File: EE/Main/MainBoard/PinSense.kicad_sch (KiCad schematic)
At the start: 15 parts, among them U10 DRV5032AJDBZR, U6 DRV5032AJDBZR, U7 DRV5032AJDBZR, U8 DRV5032AJDBZR, U9 DRV5032AJDBZR

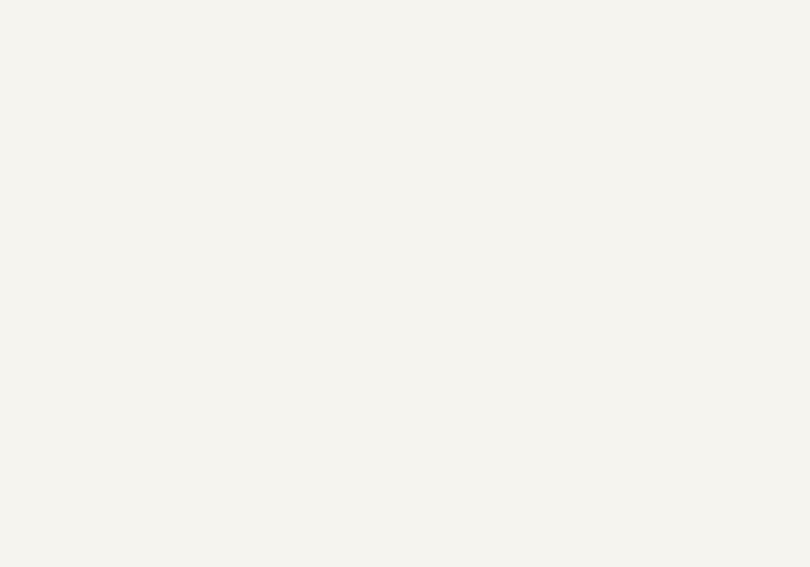
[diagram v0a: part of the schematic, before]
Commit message: Potential Revision
Potentially fabb-able rev.
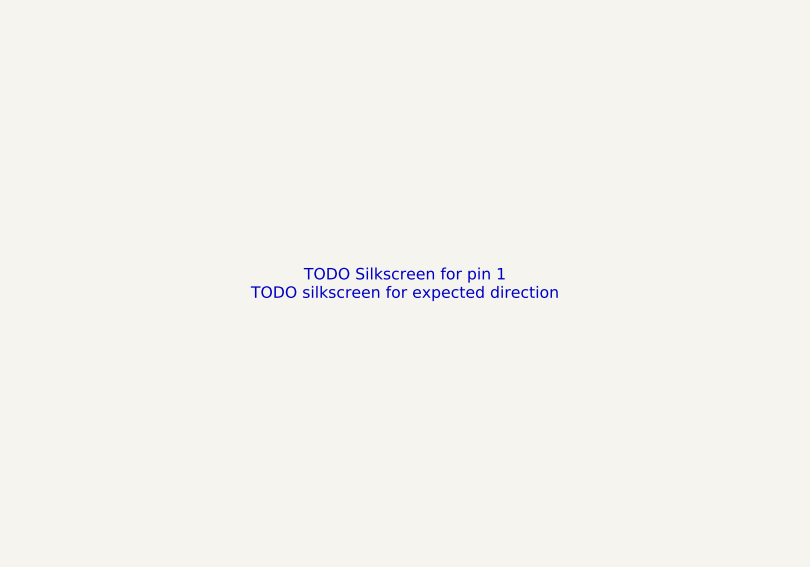
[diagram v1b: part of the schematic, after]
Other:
- note added: "TODO Silkscreen for pin 1 TODO silkscreen for expected direction"
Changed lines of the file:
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@@
 		(at 133.858 114.3)
+	)
+	(text "TODO Silkscreen for pin 1\nTODO silkscreen for expected direction"
+		(exclude_from_sim no)
+		(at 119.634 44.45 0)
+		(effects
+			(font
+				(size 1.27 1.27)
+			)
+		)
 	)
 	(label "End"

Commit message: Checkin of Fabbed Board
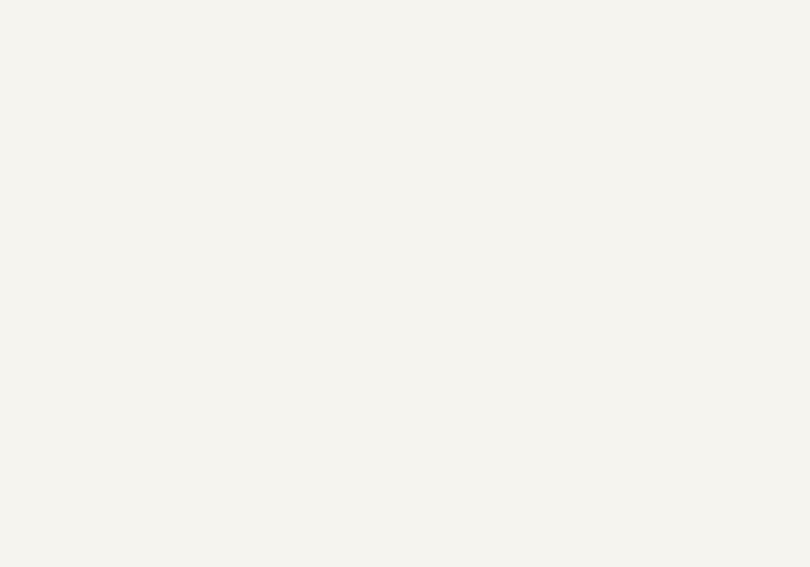
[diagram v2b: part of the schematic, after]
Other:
- note removed: "TODO Silkscreen for pin 1 TODO silkscreen for expected direction"
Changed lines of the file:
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@@
 		(at 133.858 114.3)
-	)
-	(text "TODO Silkscreen for pin 1\nTODO silkscreen for expected direction"
-		(exclude_from_sim no)
-		(at 119.634 44.45 0)
-		(effects
-			(font
-				(size 1.27 1.27)
-			)
-		)
 	)
 	(label "End"

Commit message: Updating Format, Adding Rev2 Start
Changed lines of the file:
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@@
 (kicad_sch
-	(version 20231120)
+	(version 20250114)
 	(generator "eeschema")
-	(generator_version "8.0")
+	(generator_version "9.0")
 	(paper "A4")
 	(no_connect
@@
 	(label "End"
 		(at 229.87 116.84 0)
-		(fields_autoplaced yes)
 		(effects
 			(font
@@
 	(label "Start_01"
 		(at 95.25 116.84 0)
-		(fields_autoplaced yes)
 		(effects
 			(font
@@
 	(label "Start_00"
 		(at 22.86 15.24 0)
-		(fields_autoplaced yes)
 		(effects
 			(font
@@
 	(label "Start_00"
 		(at 55.88 116.84 0)
-		(fields_autoplaced yes)
 		(effects
 			(font
@@
 	(label "Start_01"
 		(at 22.86 17.78 0)
-		(fields_autoplaced yes)
 		(effects
 			(font
@@
 	(label "Start_11"
 		(at 161.29 118.11 0)
-		(fields_autoplaced yes)
 		(effects
 			(font
@@
 	(label "End"
 		(at 22.86 25.4 0)
-		(fields_autoplaced yes)
 		(effects
 			(font
@@
 	(label "Start_10"
 		(at 129.54 118.11 0)
-		(fields_autoplaced yes)
 		(effects
 			(font
@@
 	(label "Start_10"
 		(at 22.86 20.32 0)
-		(fields_autoplaced yes)
 		(effects
 			(font
@@
 	(label "Start_11"
 		(at 22.86 22.86 0)
-		(fields_autoplaced yes)
 		(effects
 			(font
@@
 		(shape input)
 		(at 22.86 15.24 180)
-		(fields_autoplaced yes)
 		(effects
 			(font
@@
 		(shape input)
 		(at 22.86 25.4 180)
-		(fields_autoplaced yes)
 		(effects
 			(font
@@
 		(shape input)
 		(at 22.86 22.86 180)
-		(fields_autoplaced yes)
 		(effects
 			(font
@@
 		(shape input)
 		(at 22.86 20.32 180)
-		(fields_autoplaced yes)
 		(effects
 			(font
@@
 		(shape input)
 		(at 22.86 17.78 180)
-		(fields_autoplaced yes)
 		(effects
 			(font
